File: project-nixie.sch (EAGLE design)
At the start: 8 parts, among them J1 D

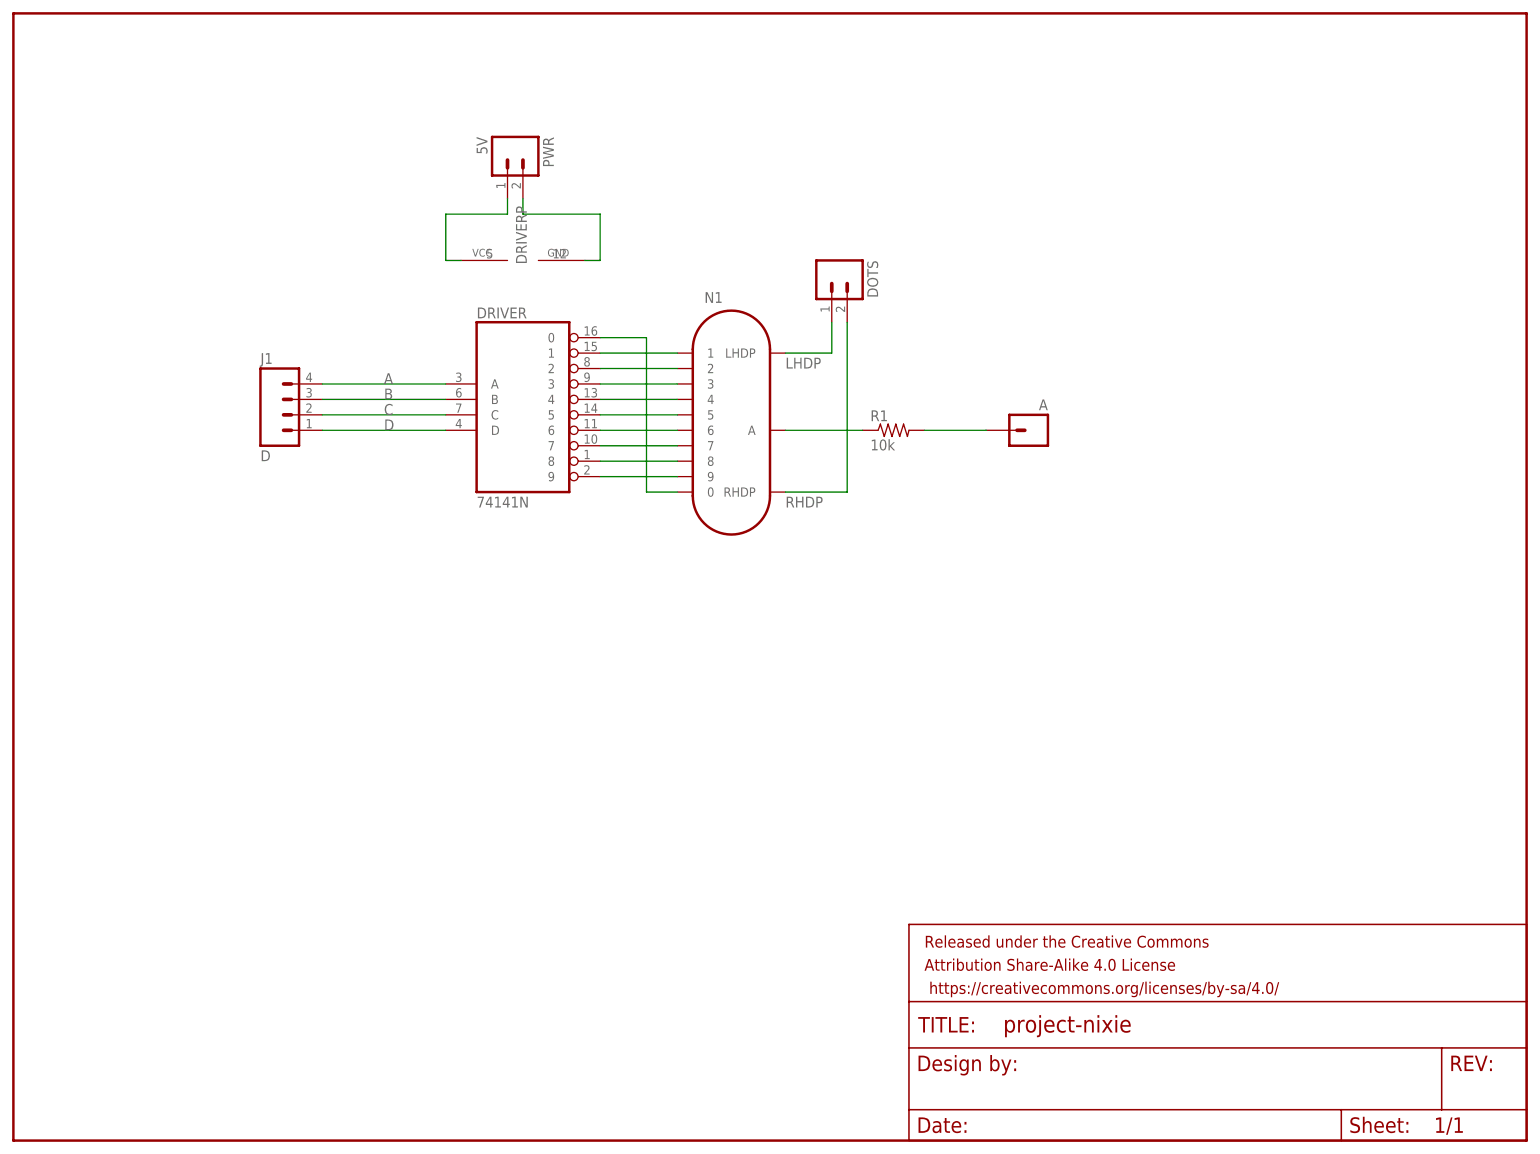
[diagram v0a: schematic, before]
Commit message: re-upload to seeed
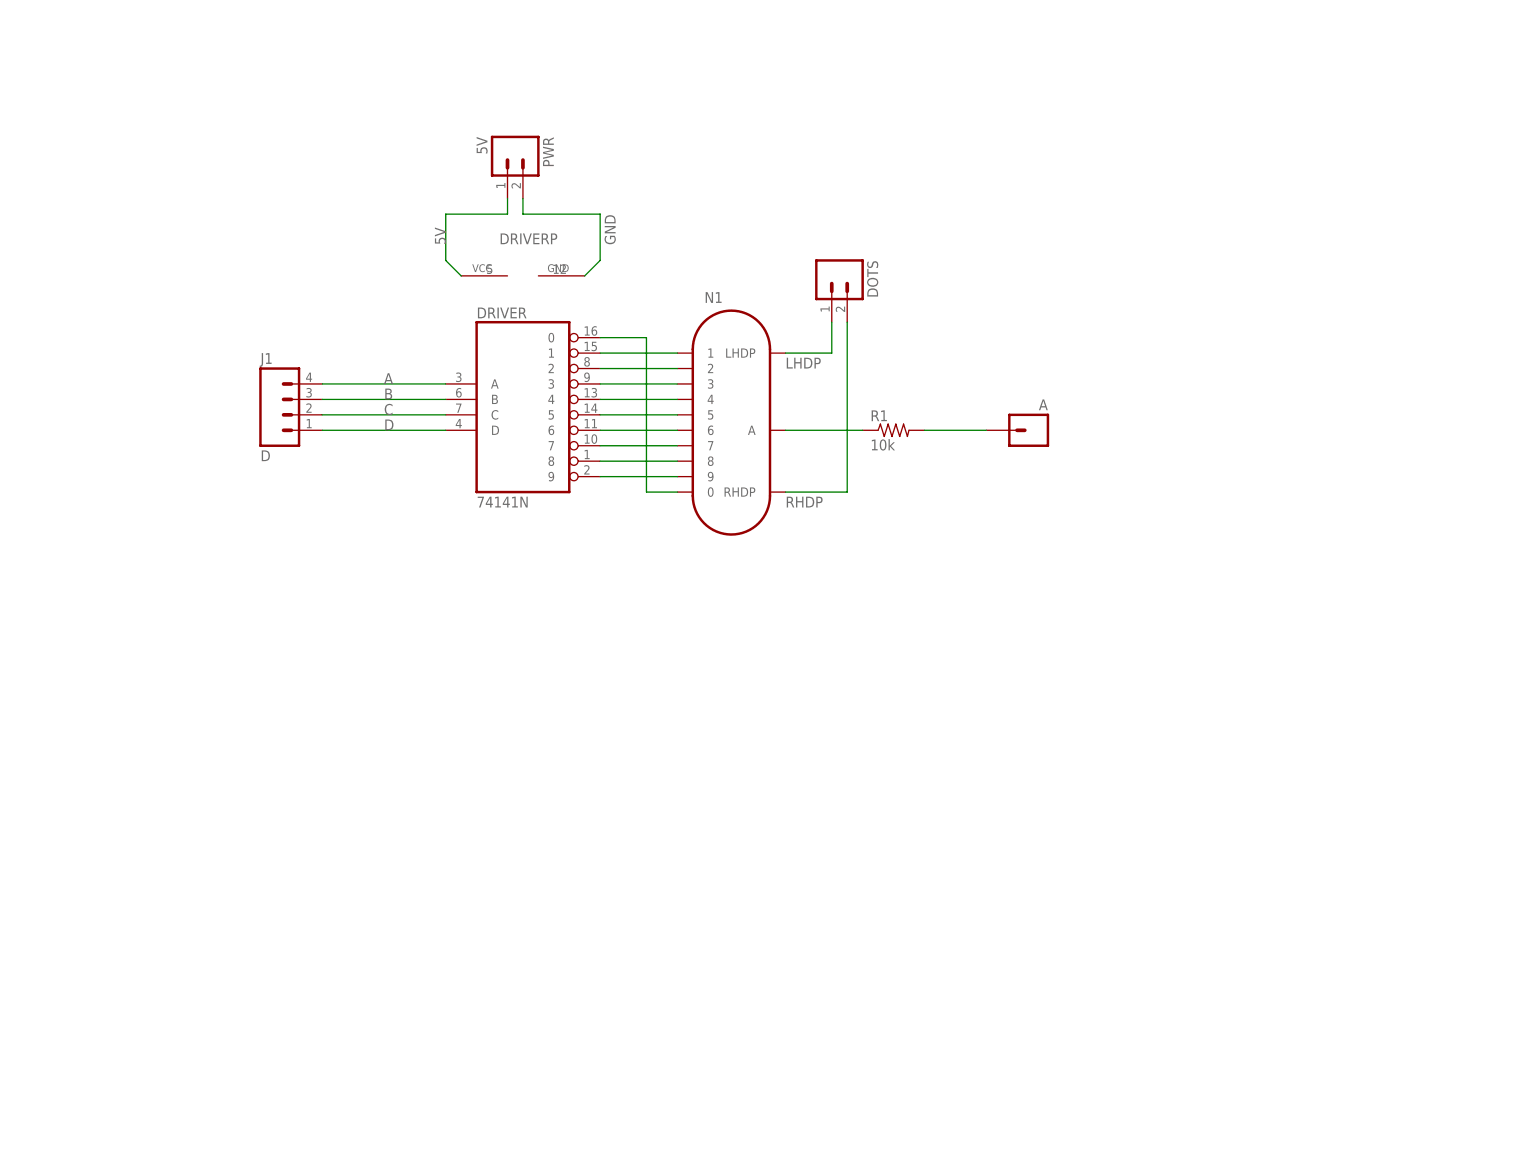
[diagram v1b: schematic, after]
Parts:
- removed FRAME1: FRAME-LETTER, SparkFun-Aesthetics:FRAME-LETTER
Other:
- moved on the sheet: DRIVERP
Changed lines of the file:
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@@
 <grid distance="0.1" unitdist="inch" unit="inch" style="lines" multiple="1" display="no" altdistance="0.01" altunitdist="inch" altunit="inch"/>
 <layers>
-<layer number="1" name="Top" color="4" fill="1" visible="yes" active="no"/>
-<layer number="16" name="Bottom" color="1" fill="1" visible="yes" active="no"/>
-<layer number="17" name="Pads" color="2" fill="1" visible="yes" active="no"/>
-<layer number="18" name="Vias" color="2" fill="1" visible="yes" active="no"/>
-<layer number="19" name="Unrouted" color="6" fill="1" visible="yes" active="no"/>
-<layer number="20" name="Dimension" color="15" fill="1" visible="yes" active="no"/>
-<layer number="21" name="tPlace" color="7" fill="1" visible="yes" active="no"/>
-<layer number="22" name="bPlace" color="7" fill="1" visible="yes" active="no"/>
-<layer number="23" name="tOrigins" color="15" fill="1" visible="yes" active="no"/>
-<layer number="24" name="bOrigins" color="15" fill="1" visible="yes" active="no"/>
-<layer number="25" name="tNames" color="7" fill="1" visible="yes" active="no"/>
-<layer number="26" name="bNames" color="7" fill="1" visible="yes" active="no"/>
-<layer number="27" name="tValues" color="7" fill="1" visible="yes" active="no"/>
-<layer number="28" name="bValues" color="7" fill="1" visible="yes" active="no"/>
+<layer number="1" name="Top" color="4" fill="1" visible="no" active="no"/>
+<layer number="16" name="Bottom" color="1" fill="1" visible="no" active="no"/>
+<layer number="17" name="Pads" color="2" fill="1" visible="no" active="no"/>
+<layer number="18" name="Vias" color="2" fill="1" visible="no" active="no"/>
+<layer number="19" name="Unrouted" color="6" fill="1" visible="no" active="no"/>
+<layer number="20" name="Dimension" color="15" fill="1" visible="no" active="no"/>
+<layer number="21" name="tPlace" color="7" fill="1" visible="no" active="no"/>
+<layer number="22" name="bPlace" color="7" fill="1" visible="no" active="no"/>
+<layer number="23" name="tOrigins" color="15" fill="1" visible="no" active="no"/>
+<layer number="24" name="bOrigins" color="15" fill="1" visible="no" active="no"/>
+<layer number="25" name="tNames" color="7" fill="1" visible="no" active="no"/>
+<layer number="26" name="bNames" color="7" fill="1" visible="no" active="no"/>
+<layer number="27" name="tValues" color="7" fill="1" visible="no" active="no"/>
+<layer number="28" name="bValues" color="7" fill="1" visible="no" active="no"/>
 <layer number="29" name="tStop" color="15" fill="3" visible="no" active="no"/>
 <layer number="30" name="bStop" color="7" fill="6" visible="no" active="no"/>
@@
 <layer number="35" name="tGlue" color="7" fill="4" visible="no" active="no"/>
 <layer number="36" name="bGlue" color="7" fill="5" visible="no" active="no"/>
-<layer number="37" name="tTest" color="7" fill="1" visible="yes" active="no"/>
-<layer number="38" name="bTest" color="7" fill="1" visible="yes" active="no"/>
+<layer number="37" name="tTest" color="7" fill="1" visible="no" active="no"/>
+<layer number="38" name="bTest" color="7" fill="1" visible="no" active="no"/>
 <layer number="39" name="tKeepout" color="4" fill="11" visible="no" active="no"/>
 <layer number="40" name="bKeepout" color="1" fill="11" visible="no" active="no"/>
@@
 <layer number="44" name="Drills" color="7" fill="1" visible="no" active="no"/>
 <layer number="45" name="Holes" color="7" fill="1" visible="no" active="no"/>
-<layer number="46" name="Milling" color="3" fill="1" visible="yes" active="no"/>
-<layer number="47" name="Measures" color="7" fill="1" visible="yes" active="no"/>
-<layer number="48" name="Document" color="7" fill="1" visible="yes" active="no"/>
-<layer number="49" name="Reference" color="13" fill="1" visible="yes" active="no"/>
-<layer number="50" name="dxf" color="7" fill="1" visible="yes" active="no"/>
-<layer number="51" name="tDocu" color="14" fill="1" visible="yes" active="no"/>
-<layer number="52" name="bDocu" color="7" fill="1" visible="yes" active="no"/>
-<layer number="53" name="tGND_GNDA" color="7" fill="9" visible="yes" active="no"/>
-<layer number="54" name="bGND_GNDA" color="1" fill="9" visible="yes" active="no"/>
-<layer number="56" name="wert" color="7" fill="1" visible="yes" active="no"/>
-<layer number="57" name="tCAD" color="7" fill="1" visible="yes" active="no"/>
-<layer number="59" name="tCarbon" color="7" fill="1" visible="yes" active="no"/>
-<layer number="60" name="bCarbon" color="7" fill="1" visible="yes" active="no"/>
+<layer number="46" name="Milling" color="3" fill="1" visible="no" active="no"/>
+<layer number="47" name="Measures" color="7" fill="1" visible="no" active="no"/>
+<layer number="48" name="Document" color="7" fill="1" visible="no" active="no"/>
+<layer number="49" name="Reference" color="13" fill="1" visible="no" active="no"/>
+<layer number="50" name="dxf" color="7" fill="1" visible="no" active="no"/>
+<layer number="51" name="tDocu" color="14" fill="1" visible="no" active="no"/>
+<layer number="52" name="bDocu" color="7" fill="1" visible="no" active="no"/>
+<layer number="53" name="tGND_GNDA" color="7" fill="9" visible="no" active="no"/>
+<layer number="54" name="bGND_GNDA" color="1" fill="9" visible="no" active="no"/>
+<layer number="56" name="wert" color="7" fill="1" visible="no" active="no"/>
+<layer number="57" name="tCAD" color="7" fill="1" visible="no" active="no"/>
+<layer number="59" name="tCarbon" color="7" fill="1" visible="no" active="no"/>
+<layer number="60" name="bCarbon" color="7" fill="1" visible="no" active="no"/>
 <layer number="90" name="Modules" color="5" fill="1" visible="yes" active="yes"/>
 <layer number="91" name="Nets" color="2" fill="1" visible="yes" active="yes"/>
@@
 </classes>
 <parts>
-<part name="FRAME1" library="SparkFun-Aesthetics" deviceset="FRAME-LETTER" device=""/>
 <part name="N1" library="russian-nixies" deviceset="IN-16" device=""/>
 <part name="DRIVER" library="74xx-us" deviceset="74*141" device="N"/>
@@
 </plain>
 <instances>
-<instance part="FRAME1" gate="G$1" x="-1549.4" y="680.72"/>
-<instance part="FRAME1" gate="V" x="-1402.08" y="680.72"/>
 <instance part="N1" gate="G$1" x="-1432.56" y="797.56"/>
 <instance part="DRIVER" gate="A" x="-1465.58" y="802.64"/>
@@
 <instance part="DOTS" gate="G$1" x="-1414.78" y="822.96" rot="R270"/>
 <instance part="A" gate="G$1" x="-1381.76" y="797.56" rot="MR0"/>
-<instance part="DRIVER" gate="P" x="-1465.58" y="825.5" rot="R90"/>
+<instance part="DRIVER" gate="P" x="-1465.58" y="822.96" smashed="yes" rot="R90">
+<attribute name="NAME" x="-1459.865" y="829.945" size="1.778" layer="95" rot="R180"/>
+</instance>
 <instance part="PWR" gate="G$1" x="-1468.12" y="843.28" rot="R270"/>
 <instance part="J1" gate="G$1" x="-1503.68" y="800.1"/>
@@
 <segment>
 <pinref part="DRIVER" gate="P" pin="VCC"/>
-<wire x1="-1475.74" y1="825.5" x2="-1478.28" y2="825.5" width="0.1524" layer="91"/>
+<wire x1="-1475.74" y1="822.96" x2="-1478.28" y2="825.5" width="0.1524" layer="91"/>
 <wire x1="-1478.28" y1="825.5" x2="-1478.28" y2="833.12" width="0.1524" layer="91"/>
 <pinref part="PWR" gate="G$1" pin="1"/>
 <wire x1="-1478.28" y1="833.12" x2="-1468.12" y2="833.12" width="0.1524" layer="91"/>
 <wire x1="-1468.12" y1="833.12" x2="-1468.12" y2="835.66" width="0.1524" layer="91"/>
+<label x="-1478.28" y="828.04" size="1.778" layer="95" rot="R90"/>
 </segment>
 </net>
@@
 <segment>
 <pinref part="DRIVER" gate="P" pin="GND"/>
-<wire x1="-1455.42" y1="825.5" x2="-1452.88" y2="825.5" width="0.1524" layer="91"/>
+<wire x1="-1455.42" y1="822.96" x2="-1452.88" y2="825.5" width="0.1524" layer="91"/>
 <wire x1="-1452.88" y1="825.5" x2="-1452.88" y2="833.12" width="0.1524" layer="91"/>
 <pinref part="PWR" gate="G$1" pin="2"/>
 <wire x1="-1452.88" y1="833.12" x2="-1465.58" y2="833.12" width="0.1524" layer="91"/>
 <wire x1="-1465.58" y1="833.12" x2="-1465.58" y2="835.66" width="0.1524" layer="91"/>
-</segment>
-</net>
+<label x="-1450.34" y="828.04" size="1.778" layer="95" rot="R90"/>
+</segment>
+</net>
